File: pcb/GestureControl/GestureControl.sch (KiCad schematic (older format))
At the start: 69 parts, among them J1 Conn_01x04_I2I-LCD, J2 BATT, J3 Conn_01x08, J4 Conn_01x06, J5 Conn_01x10, J6 Conn_01x08, SW1 SW1, SW2 SW2, U1 AP5100_3.3, U2 AP5100_3.3

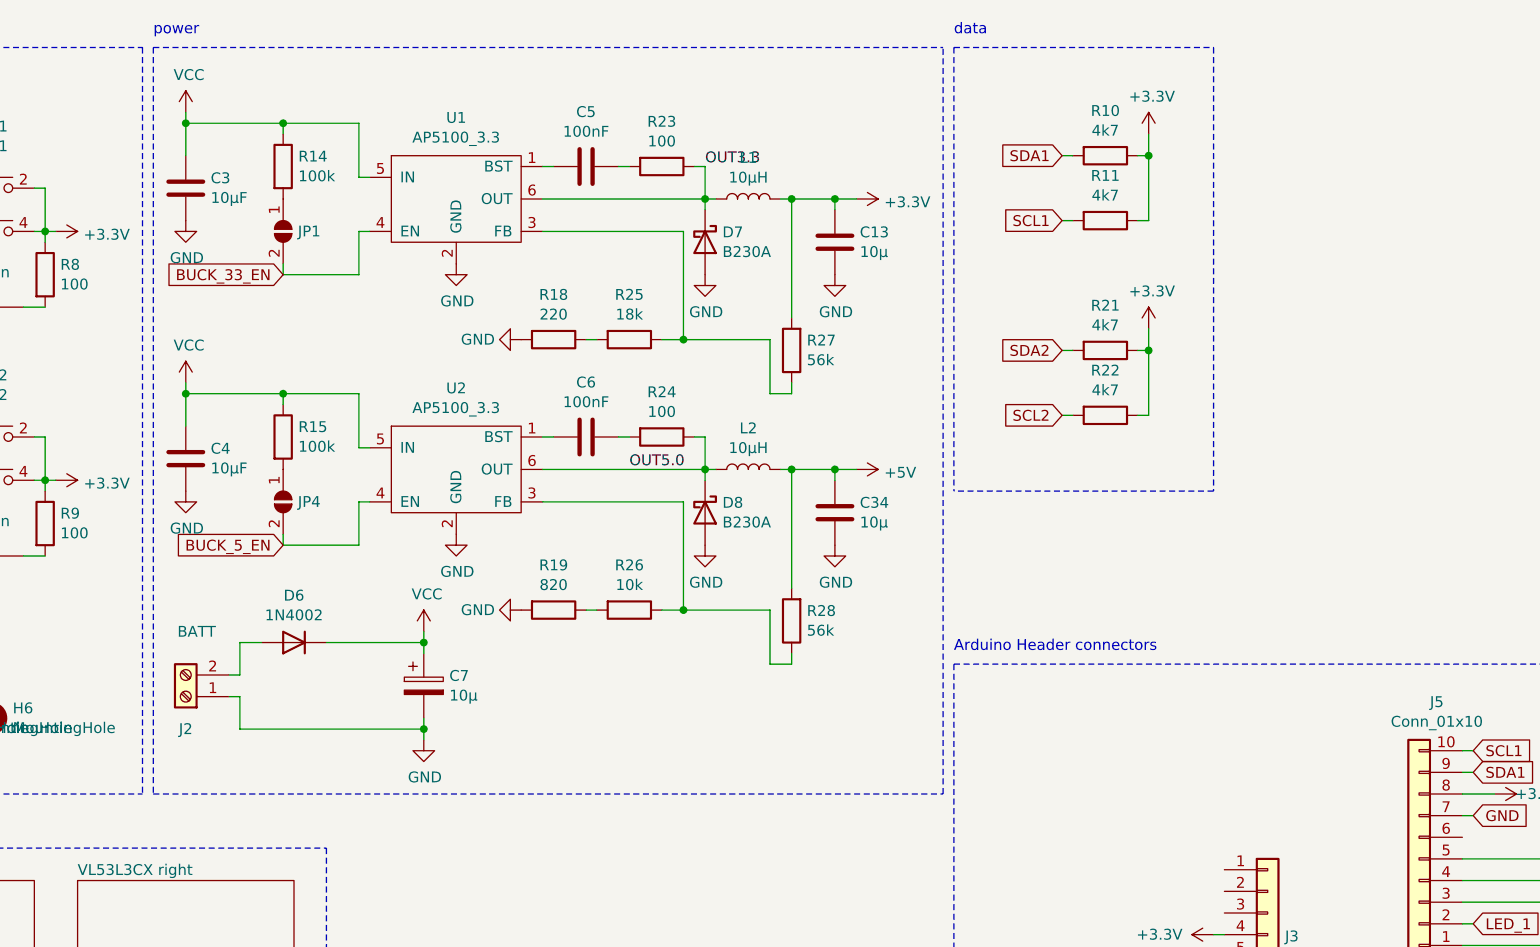
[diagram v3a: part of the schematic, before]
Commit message: update board design
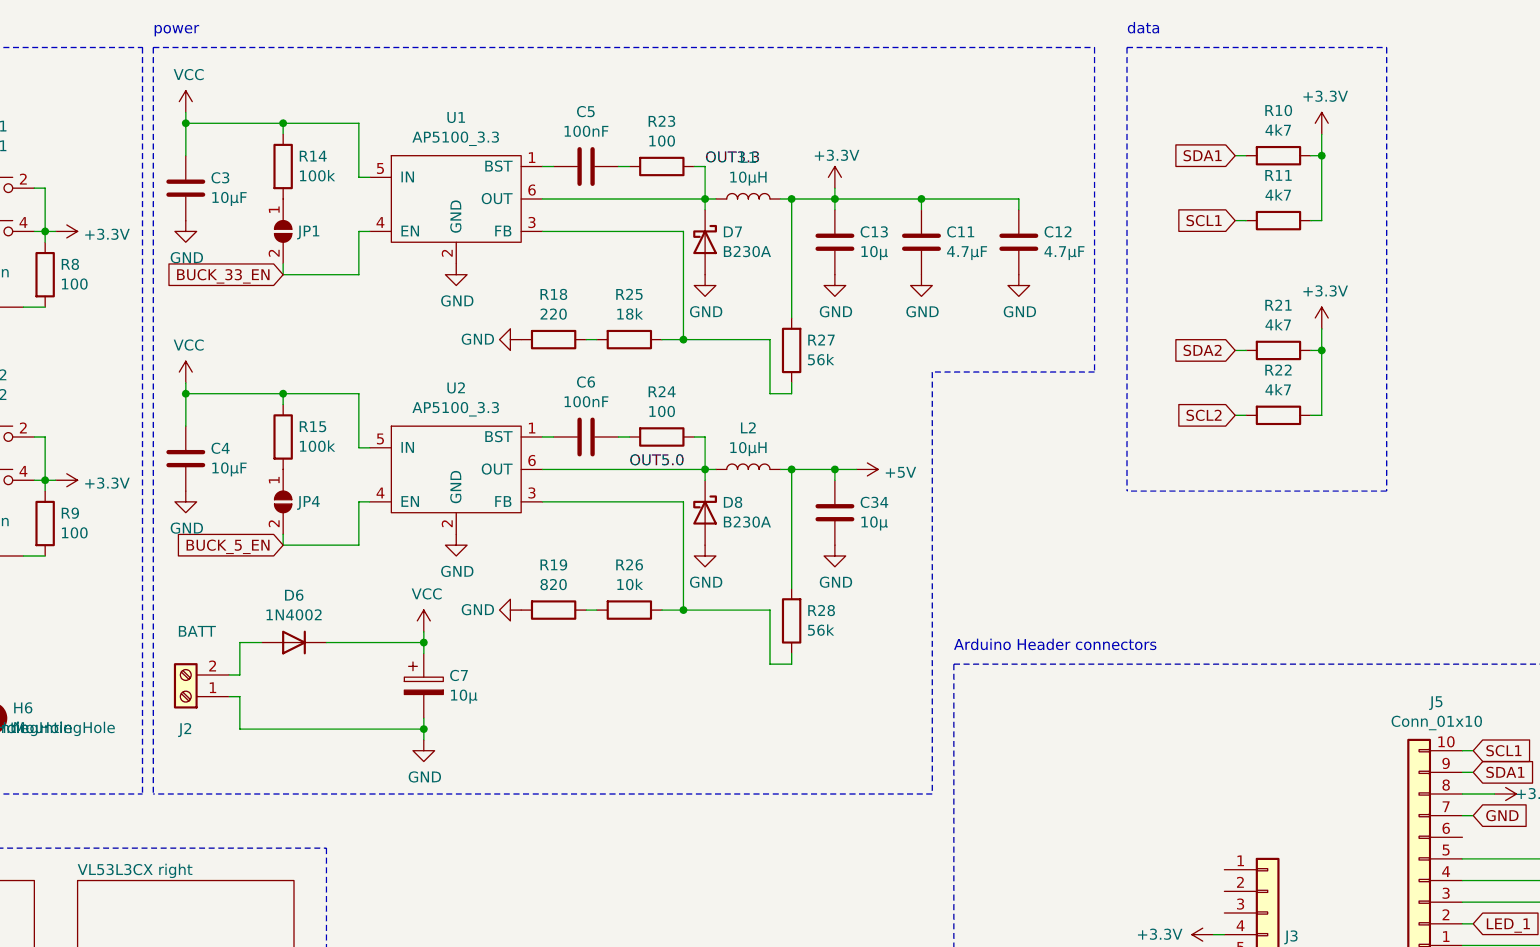
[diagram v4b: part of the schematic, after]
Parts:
- added C11, C12: 4.7µF, Capacitor_SMD:C_0805_2012Metric_Pad1.18x1.45mm_HandSolder, symbol Device:C
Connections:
- net +3V3: now also C11.1, C12.1
- net GND: now also C11.2, C12.2
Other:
- moved on the sheet: R10, R11, R21, R22
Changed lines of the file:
@@
 Wire Wire Line
 	8500 5500 8450 5500
-Text GLabel 7750 1250 0    50   Input ~ 0
+Text GLabel 8550 1250 0    50   Input ~ 0
 SDA1
-Text GLabel 7750 1550 0    50   Input ~ 0
+Text GLabel 8550 1550 0    50   Input ~ 0
 SCL1
 Wire Wire Line
-	7750 1550 7800 1550
-Wire Wire Line
-	7800 1250 7750 1250
+	8550 1550 8600 1550
+Wire Wire Line
+	8600 1250 8550 1250
 $Comp
 L power:+3.3V #PWR016
 U 1 1 62142CB7
-P 8150 1150
-F 0 "#PWR016" H 8150 1000 50  0001 C CNN
-F 1 "+3.3V" H 8165 1323 50  0000 C CNN
-F 2 "" H 8150 1150 50  0001 C CNN
-F 3 "" H 8150 1150 50  0001 C CNN
-	1    8150 1150
-	1    0    0    -1
-$EndComp
-Wire Wire Line
-	8150 1150 8150 1250
-Wire Wire Line
-	8150 1250 8100 1250
-Wire Wire Line
-	8100 1550 8150 1550
-Wire Wire Line
-	8150 1550 8150 1250
-Connection ~ 8150 1250
+P 8950 1150
+F 0 "#PWR016" H 8950 1000 50  0001 C CNN
+F 1 "+3.3V" H 8965 1323 50  0000 C CNN
+F 2 "" H 8950 1150 50  0001 C CNN
+F 3 "" H 8950 1150 50  0001 C CNN
+	1    8950 1150
+	1    0    0    -1
+$EndComp
+Wire Wire Line
+	8950 1150 8950 1250
+Wire Wire Line
+	8950 1250 8900 1250
+Wire Wire Line
+	8900 1550 8950 1550
+Wire Wire Line
+	8950 1550 8950 1250
+Connection ~ 8950 1250
 $Comp
 L Device:R R11
 U 1 1 6213D612
-P 7950 1550
-F 0 "R11" V 7743 1550 50  0000 C CNN
-F 1 "4k7" V 7834 1550 50  0000 C CNN
-F 2 "Resistor_SMD:R_0805_2012Metric_Pad1.20x1.40mm_HandSolder" V 7880 1550 50  0001 C CNN
-F 3 "~" H 7950 1550 50  0001 C CNN
-	1    7950 1550
+P 8750 1550
+F 0 "R11" V 8543 1550 50  0000 C CNN
+F 1 "4k7" V 8634 1550 50  0000 C CNN
+F 2 "Resistor_SMD:R_0805_2012Metric_Pad1.20x1.40mm_HandSolder" V 8680 1550 50  0001 C CNN
+F 3 "~" H 8750 1550 50  0001 C CNN
+	1    8750 1550
 	0    1    1    0
 $EndComp
@@
 L Device:R R10
 U 1 1 6213CF4B
-P 7950 1250
-F 0 "R10" V 7743 1250 50  0000 C CNN
-F 1 "4k7" V 7834 1250 50  0000 C CNN
-F 2 "Resistor_SMD:R_0805_2012Metric_Pad1.20x1.40mm_HandSolder" V 7880 1250 50  0001 C CNN
-F 3 "~" H 7950 1250 50  0001 C CNN
-	1    7950 1250
+P 8750 1250
+F 0 "R10" V 8543 1250 50  0000 C CNN
+F 1 "4k7" V 8634 1250 50  0000 C CNN
+F 2 "Resistor_SMD:R_0805_2012Metric_Pad1.20x1.40mm_HandSolder" V 8680 1250 50  0001 C CNN
+F 3 "~" H 8750 1250 50  0001 C CNN
+	1    8750 1250
 	0    1    1    0
 $EndComp
@@
 Arduino Header connectors
 Wire Notes Line
-	7250 750  8450 750
-Text Notes 7250 700  0    50   ~ 0
+	8050 750  9250 750
+Text Notes 8050 700  0    50   ~ 0
 data
 Text Notes 700  4400 0    50   ~ 0
@@
 F1 "STM32L151RET6TR.sch" 50
 $EndSheet
-Text GLabel 7750 2150 0    50   Input ~ 0
+Text GLabel 8550 2150 0    50   Input ~ 0
 SDA2
-Text GLabel 7750 2450 0    50   Input ~ 0
+Text GLabel 8550 2450 0    50   Input ~ 0
 SCL2
 Wire Wire Line
-	7750 2450 7800 2450
-Wire Wire Line
-	7800 2150 7750 2150
+	8550 2450 8600 2450
+Wire Wire Line
+	8600 2150 8550 2150
 $Comp
 L power:+3.3V #PWR0103
 U 1 1 62898F4E
-P 8150 2050
-F 0 "#PWR0103" H 8150 1900 50  0001 C CNN
-F 1 "+3.3V" H 8165 2223 50  0000 C CNN
-F 2 "" H 8150 2050 50  0001 C CNN
-F 3 "" H 8150 2050 50  0001 C CNN
-	1    8150 2050
-	1    0    0    -1
-$EndComp
-Wire Wire Line
-	8150 2050 8150 2150
-Wire Wire Line
-	8150 2150 8100 2150
-Wire Wire Line
-	8100 2450 8150 2450
-Wire Wire Line
-	8150 2450 8150 2150
-Connection ~ 8150 2150
+P 8950 2050
+F 0 "#PWR0103" H 8950 1900 50  0001 C CNN
+F 1 "+3.3V" H 8965 2223 50  0000 C CNN
+F 2 "" H 8950 2050 50  0001 C CNN
+F 3 "" H 8950 2050 50  0001 C CNN
+	1    8950 2050
+	1    0    0    -1
+$EndComp
+Wire Wire Line
+	8950 2050 8950 2150
+Wire Wire Line
+	8950 2150 8900 2150
+Wire Wire Line
+	8900 2450 8950 2450
+Wire Wire Line
+	8950 2450 8950 2150
+Connection ~ 8950 2150
 $Comp
 L Device:R R22
 U 1 1 62898F59
-P 7950 2450
-F 0 "R22" V 7743 2450 50  0000 C CNN
-F 1 "4k7" V 7834 2450 50  0000 C CNN
-F 2 "Resistor_SMD:R_0805_2012Metric_Pad1.20x1.40mm_HandSolder" V 7880 2450 50  0001 C CNN
-F 3 "~" H 7950 2450 50  0001 C CNN
-	1    7950 2450
+P 8750 2450
+F 0 "R22" V 8543 2450 50  0000 C CNN
+F 1 "4k7" V 8634 2450 50  0000 C CNN
+F 2 "Resistor_SMD:R_0805_2012Metric_Pad1.20x1.40mm_HandSolder" V 8680 2450 50  0001 C CNN
+F 3 "~" H 8750 2450 50  0001 C CNN
+	1    8750 2450
 	0    1    1    0
 $EndComp
@@
 L Device:R R21
 U 1 1 62898F5F
-P 7950 2150
-F 0 "R21" V 7743 2150 50  0000 C CNN
-F 1 "4k7" V 7834 2150 50  0000 C CNN
-F 2 "Resistor_SMD:R_0805_2012Metric_Pad1.20x1.40mm_HandSolder" V 7880 2150 50  0001 C CNN
-F 3 "~" H 7950 2150 50  0001 C CNN
-	1    7950 2150
-	0    1    1    0
-$EndComp
-Wire Notes Line
-	8450 2800 7250 2800
-Wire Notes Line
-	8450 750  8450 2800
-Wire Notes Line
-	7250 750  7250 2800
+P 8750 2150
+F 0 "R21" V 8543 2150 50  0000 C CNN
+F 1 "4k7" V 8634 2150 50  0000 C CNN
+F 2 "Resistor_SMD:R_0805_2012Metric_Pad1.20x1.40mm_HandSolder" V 8680 2150 50  0001 C CNN
+F 3 "~" H 8750 2150 50  0001 C CNN
+	1    8750 2150
+	0    1    1    0
+$EndComp
+Wire Notes Line
+	9250 2800 8050 2800
+Wire Notes Line
+	9250 750  9250 2800
+Wire Notes Line
+	8050 750  8050 2800
 Wire Notes Line
 	2000 5850 2000 6850
@@
 L power:+3.3V #PWR0120
 U 1 1 62250C10
-P 6800 1450
-F 0 "#PWR0120" H 6800 1300 50  0001 C CNN
-F 1 "+3.3V" V 6815 1578 50  0000 L CNN
-F 2 "" H 6800 1450 50  0001 C CNN
-F 3 "" H 6800 1450 50  0001 C CNN
-	1    6800 1450
-	0    1    1    0
+P 6700 1400
+F 0 "#PWR0120" H 6700 1250 50  0001 C CNN
+F 1 "+3.3V" H 6600 1550 50  0000 L CNN
+F 2 "" H 6700 1400 50  0001 C CNN
+F 3 "" H 6700 1400 50  0001 C CNN
+	1    6700 1400
+	1    0    0    -1
 $EndComp
 $Comp
@@
 Wire Wire Line
 	6450 1450 6500 1450
-Wire Wire Line
-	6800 1450 6700 1450
 Connection ~ 6700 1450
 Connection ~ 6500 1450
@@
 $EndComp
 Wire Notes Line
-	3550 4200 7200 4200
-Wire Notes Line
-	7200 4200 7200 750
-Wire Notes Line
 	3550 750  3550 4200
-Wire Notes Line
-	3550 750  7200 750
 Wire Wire Line
 	9600 4200 9750 4200
@@
 Wire Notes Line
 	7250 3600 7250 6500
+$Comp
+L Device:C C11
+U 1 1 62216B61
+P 7100 1650
+F 0 "C11" H 7215 1696 50  0000 L CNN
+F 1 "4.7µF" H 7215 1605 50  0000 L CNN
+F 2 "Capacitor_SMD:C_0805_2012Metric_Pad1.18x1.45mm_HandSolder" H 7138 1500 50  0001 C CNN
+F 3 "~" H 7100 1650 50  0001 C CNN
+	1    7100 1650
+	1    0    0    -1
+$EndComp
+$Comp
+L Device:C C12
+U 1 1 6222AC8B
+P 7550 1650
+F 0 "C12" H 7665 1696 50  0000 L CNN
+F 1 "4.7µF" H 7665 1605 50  0000 L CNN
+F 2 "Capacitor_SMD:C_0805_2012Metric_Pad1.18x1.45mm_HandSolder" H 7588 1500 50  0001 C CNN
+F 3 "~" H 7550 1650 50  0001 C CNN
+	1    7550 1650
+	1    0    0    -1
+$EndComp
+Wire Wire Line
+	6700 1400 6700 1450
+Wire Wire Line
+	7100 1450 7100 1500
+Wire Wire Line
+	6700 1450 7100 1450
+Wire Wire Line
+	7100 1450 7550 1450
+Wire Wire Line
+	7550 1450 7550 1500
+Connection ~ 7100 1450
+$Comp
+L power:GND #PWR0198
+U 1 1 62262C04
+P 7100 1800
+F 0 "#PWR0198" H 7100 1550 50  0001 C CNN
+F 1 "GND" H 7105 1627 50  0000 C CNN
+F 2 "" H 7100 1800 50  0001 C CNN
+F 3 "" H 7100 1800 50  0001 C CNN
+	1    7100 1800
+	1    0    0    -1
+$EndComp
+$Comp
+L power:GND #PWR0199
+U 1 1 62263181
+P 7550 1800
+F 0 "#PWR0199" H 7550 1550 50  0001 C CNN
+F 1 "GND" H 7555 1627 50  0000 C CNN
+F 2 "" H 7550 1800 50  0001 C CNN
+F 3 "" H 7550 1800 50  0001 C CNN
+	1    7550 1800
+	1    0    0    -1
+$EndComp
+Wire Notes Line
+	3550 750  7900 750
+Wire Notes Line
+	7900 2250 7150 2250
+Wire Notes Line
+	7150 2250 7150 4200
+Wire Notes Line
+	7900 750  7900 2250
+Wire Notes Line
+	7150 4200 3550 4200
 $EndSCHEMATC
